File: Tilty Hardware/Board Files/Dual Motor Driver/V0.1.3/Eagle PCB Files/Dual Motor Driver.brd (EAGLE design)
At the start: 38.4 x 50.8 mm, 43 parts, among them J1 AVR_SPI_PRG_62X3_LOCK, Q1 16MHz, U1 ATMEGA328P, U2 L298_BRIDGE_DRIVER, U3 LM2931

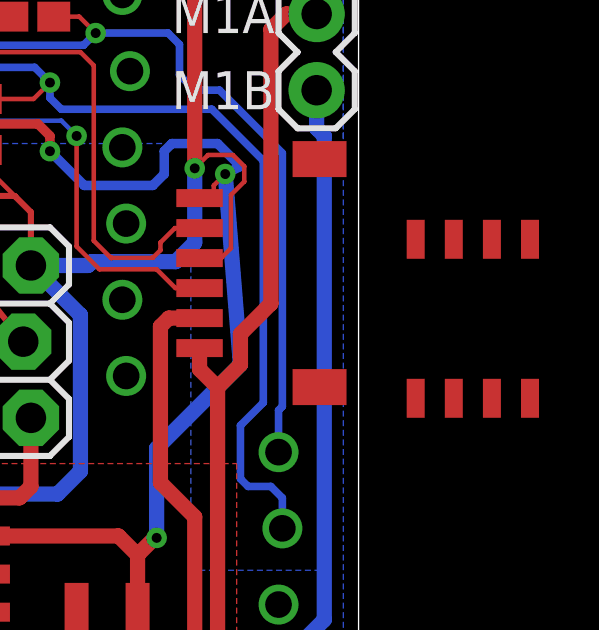
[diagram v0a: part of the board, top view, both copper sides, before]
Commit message: Updated RC adapter things.todo
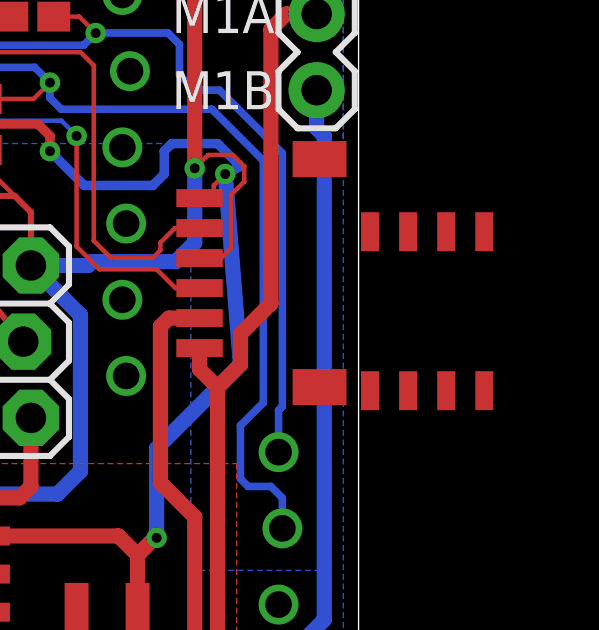
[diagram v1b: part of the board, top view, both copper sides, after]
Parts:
- moved U$1 1.55 mm to (40.6, 33.8)
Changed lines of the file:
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@@
 <attribute name="VALUE" x="5.588" y="5.08" size="1.27" layer="27"/>
 </element>
-<element name="U$1" library="My Parts" package="SOIC-8" value="PCA9306" x="42.164" y="33.528" rot="R90"/>
+<element name="U$1" library="My Parts" package="SOIC-8" value="PCA9306" x="40.64" y="33.782" rot="R90"/>
 </elements>
 <signals>
